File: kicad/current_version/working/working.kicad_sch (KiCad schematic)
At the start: 1 part, among them J1 scuath

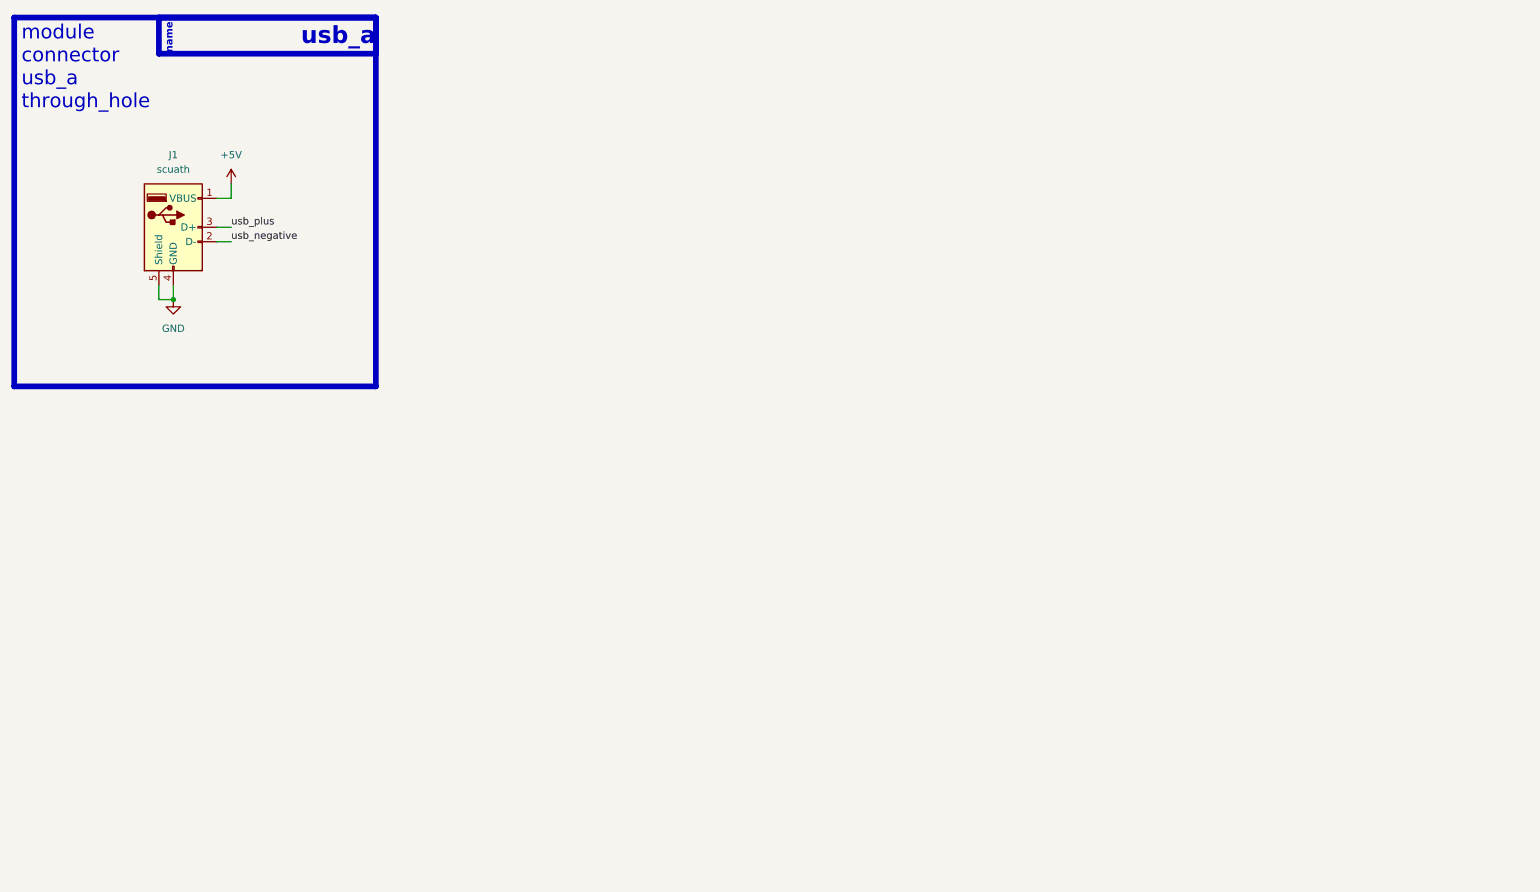
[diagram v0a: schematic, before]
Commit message: first version maybe
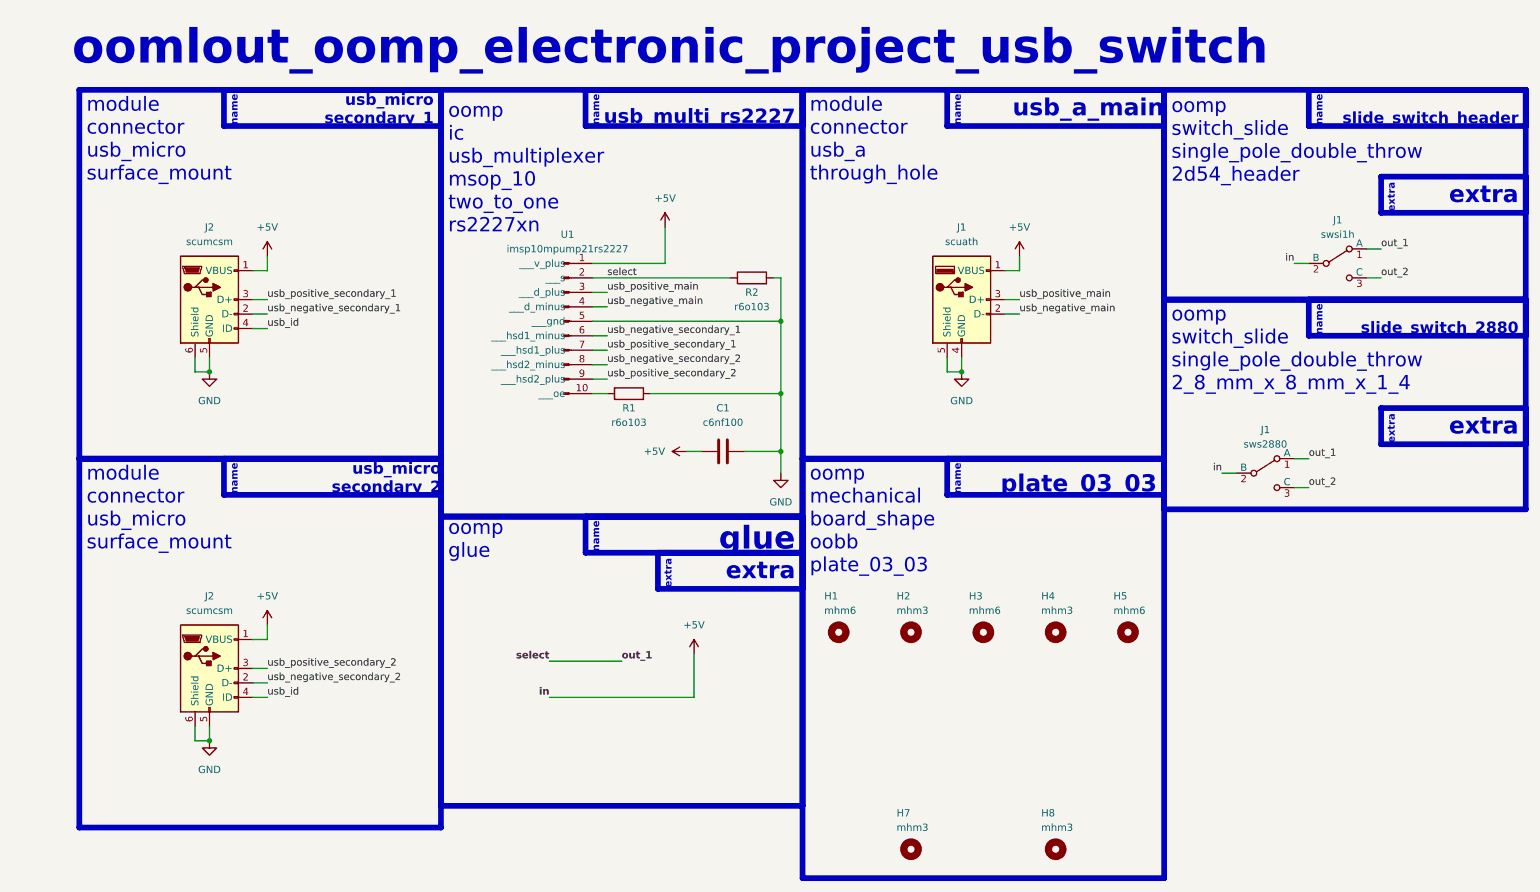
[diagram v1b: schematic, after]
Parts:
- added C1: c6nf100, oomlout_oomp_part_footprints:c6nf100_electronic_capacitor_0603_100_nano_farad, symbol oomlout_oomp_part_symbols:c6nf100_electronic_capacitor_0603_100_nano_farad
- added H1, H3, H5: mhm6, oomlout_oomp_part_footprints:mhm6_electronic_mounting_hole_m6, symbol oomlout_oomp_part_symbols:mhm6_electronic_mounting_hole_m6
- added H2, H4, H7, H8: mhm3, oomlout_oomp_part_footprints:mhm3_electronic_mounting_hole_m3, symbol oomlout_oomp_part_symbols:mhm3_electronic_mounting_hole_m3
- added J1: swsi1h, all_the_kicad_footprints_one_library:kicad_connector_pinheader_2_54mm_pinheader_1x03_p2_54mm_vertical, symbol oomlout_oomp_part_symbols:swsi1h_electronic_switch_slide_2d54_header_single_pol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
- added J1: sws2880, oomlout_oomp_part_footprints:sws2880_electronic_switch_slide_2_8_mm_x_8_mm_x_1_4_single_pole_double_throw, symbol oomlout_oomp_part_symbols:sws2880_electronic_switch_slide_2_8_mm_x_8_mm_x_1_4_s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
- added J2 (x2): scumcsm, oomlout_oomp_part_footprints:scumcsm_electronic_socket_usb_micro_surface_mount, symbol oomlout_oomp_part_symbols:scumcsm_electronic_socket_usb_micro_surface_mount
- added R1, R2: r6o103, oomlout_oomp_part_footprints:r6o103_electronic_resistor_0603_10000_ohm, symbol oomlout_oomp_part_symbols:r6o103_electronic_resistor_0603_10000_ohm
- added U1: imsp10mpump21rs2227, oomlout_oomp_part_footprints:imsp10mpump21rs2227_electronic_ic_msop_10_multiplexer_usb_multiplexer_two_to_one_jiangsu_r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, symbol oomlout_oomp_part_symbols:imsp10mpump21rs2227_electronic_ic_msop_10_multiplexer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
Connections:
- net +5V: now also C1.1, J1.2 (B), J1.2 (B), J2.1 (VBUS), J2.1 (VBUS), U1.1 (___v_plus)
- net GND: now also C1.2, J2.5 (GND), J2.5 (GND), J2.6 (Shield), J2.6 (Shield), R1.2, R2.2, U1.5 (___gnd)
- net usb_negative renamed usb_negative_main
- net usb_negative_main: now also U1.4 (___d_minus)
- net usb_plus renamed usb_positive_main
- net usb_positive_main: now also U1.3 (___d_plus)
- new net: R1.1, U1.10 (___oe)
- new net out_1: J1.1 (A), J1.1 (A), R2.1, U1.2 (___s)
- new net out_2: J1.3 (C), J1.3 (C)
- new net usb_id: J2.4 (ID), J2.4 (ID)
- new net usb_negative_secondary_1: J2.2 (D-), U1.6 (___hsd1_minus)
- new net usb_negative_secondary_2: J2.2 (D-), U1.8 (___hsd2_minus)
- new net usb_positive_secondary_1: J2.3 (D+), U1.7 (___hsd1_plus)
- new net usb_positive_secondary_2: J2.3 (D+), U1.9 (___hsd2_plus)
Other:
- note added: "extra"
- note added: "glue"
- note added: "module connector usb_micro surface_mount"
- note added: "oomlout_oomp_electronic_project_usb_switch"
- note added: "oomp glue"
- note added: "oomp ic usb_multiplexer msop_10 two_to_one rs2227xn"
- note added: "oomp mechanical board_shape oobb plate_03_03"
- note added: "oomp switch_slide single_pole_double_throw 2_8_mm_x_8_mm_x_1_4"
- note added: "oomp switch_slide single_pole_double_throw 2d54_header"
- note added: "plate_03_03"
- note added: "slide_switch_2880"
- note added: "slide_switch_header"
- note added: "usb_a_main"
- note added: "usb_micro secondary_1"
- note added: "usb_micro secondary_2"
- note added: "usb_multi_rs2227"
- note removed: "usb_a"
